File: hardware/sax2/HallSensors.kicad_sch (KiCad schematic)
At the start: 2 parts, among them J1301 2x05_Horizontal

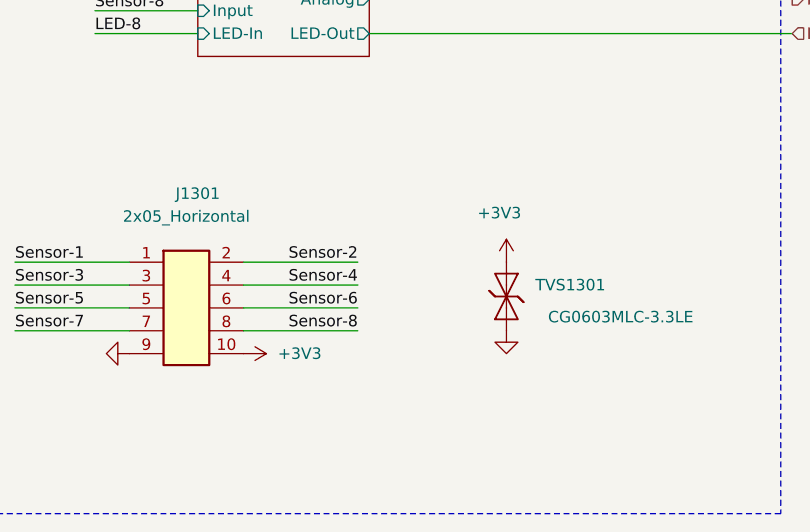
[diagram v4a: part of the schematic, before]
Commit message: Update
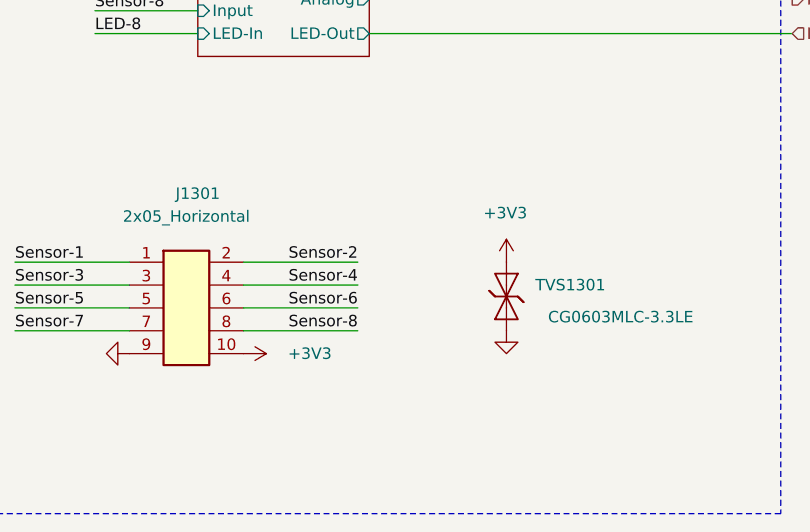
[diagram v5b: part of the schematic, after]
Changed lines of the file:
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@@
 		(on_board yes)
 		(dnp no)
-		(fields_autoplaced yes)
 		(property "Reference" "#PWR1304"
 			(at 134.62 162.56 0)
@@
 		)
 		(property "Value" "+3V3"
-			(at 142.24 162.5599 90)
-			(effects
-				(font
-					(size 1.27 1.27)
-				)
-				(justify left)
+			(at 145.796 162.5599 90)
+			(effects
+				(font
+					(size 1.27 1.27)
+					(color 255 92 187 1)
+				)
 			)
 		)
@@
 		)
 		(property "Value" "+3V3"
-			(at 169.291 146.939 0)
-			(effects
-				(font
-					(size 1.27 1.27)
-				)
-				(justify left)
-			)
-		)
+			(at 167.513 146.939 0)
+			(effects
+				(font
+					(size 1.27 1.27)
+					(color 255 92 187 1)
+				)
+			)
+		)
